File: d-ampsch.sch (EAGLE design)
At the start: 20 parts

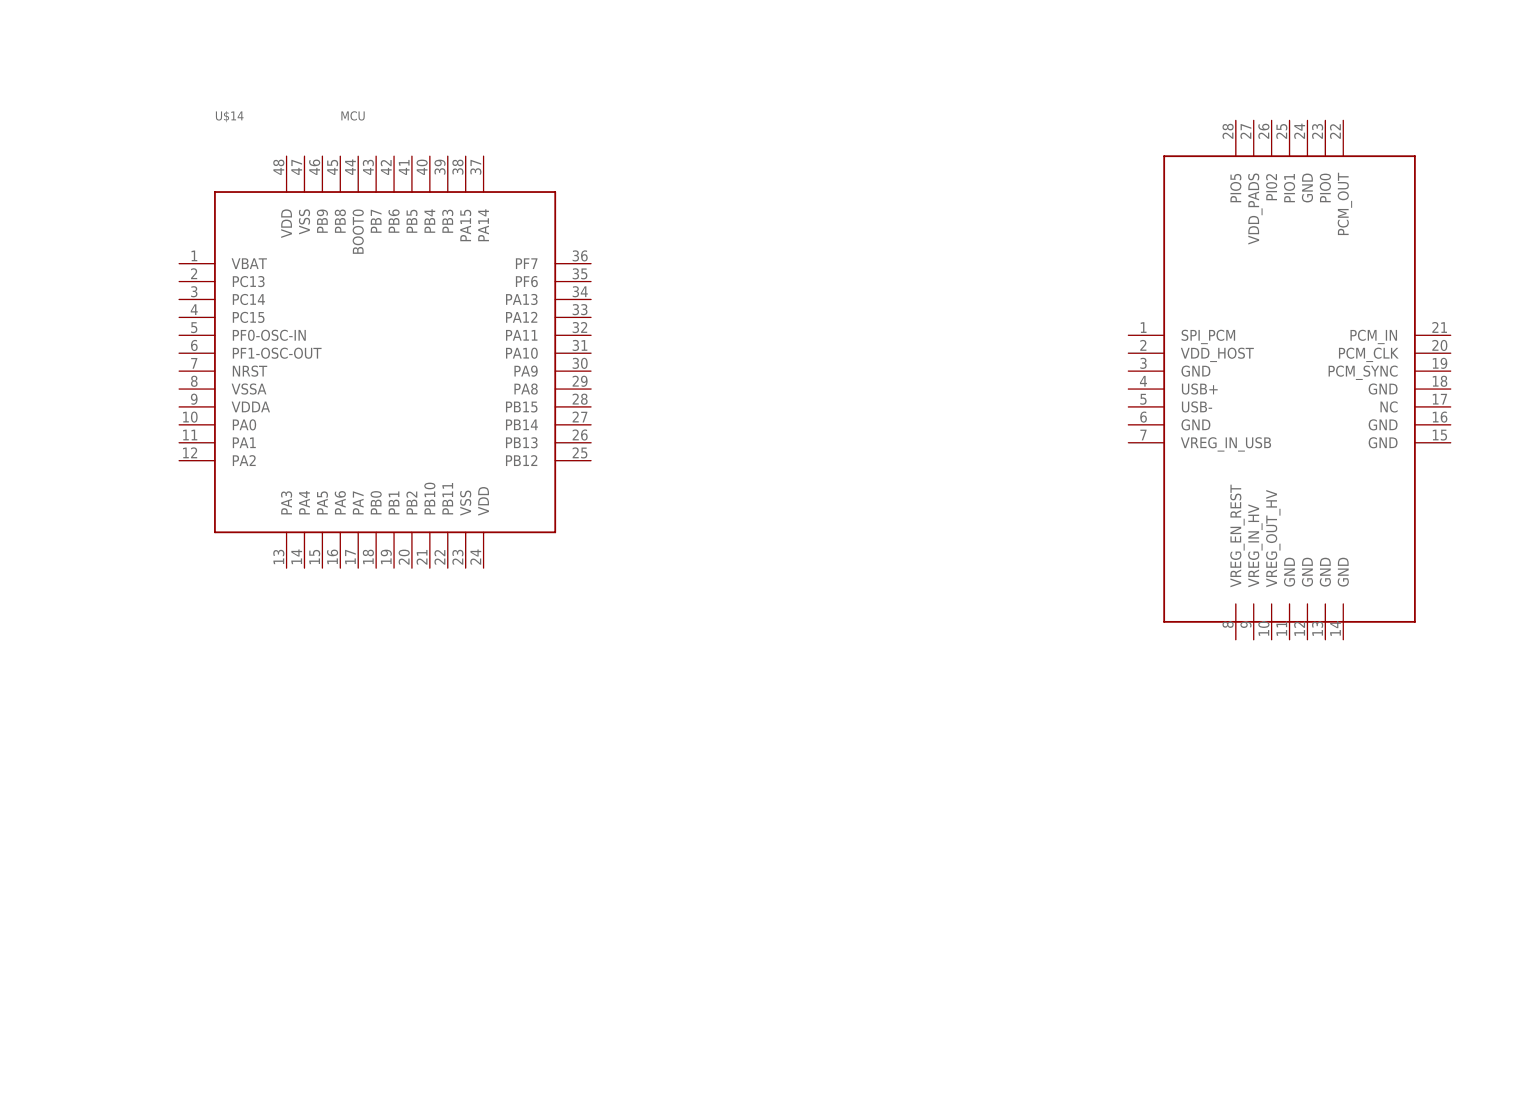
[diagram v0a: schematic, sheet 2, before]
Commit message: updates
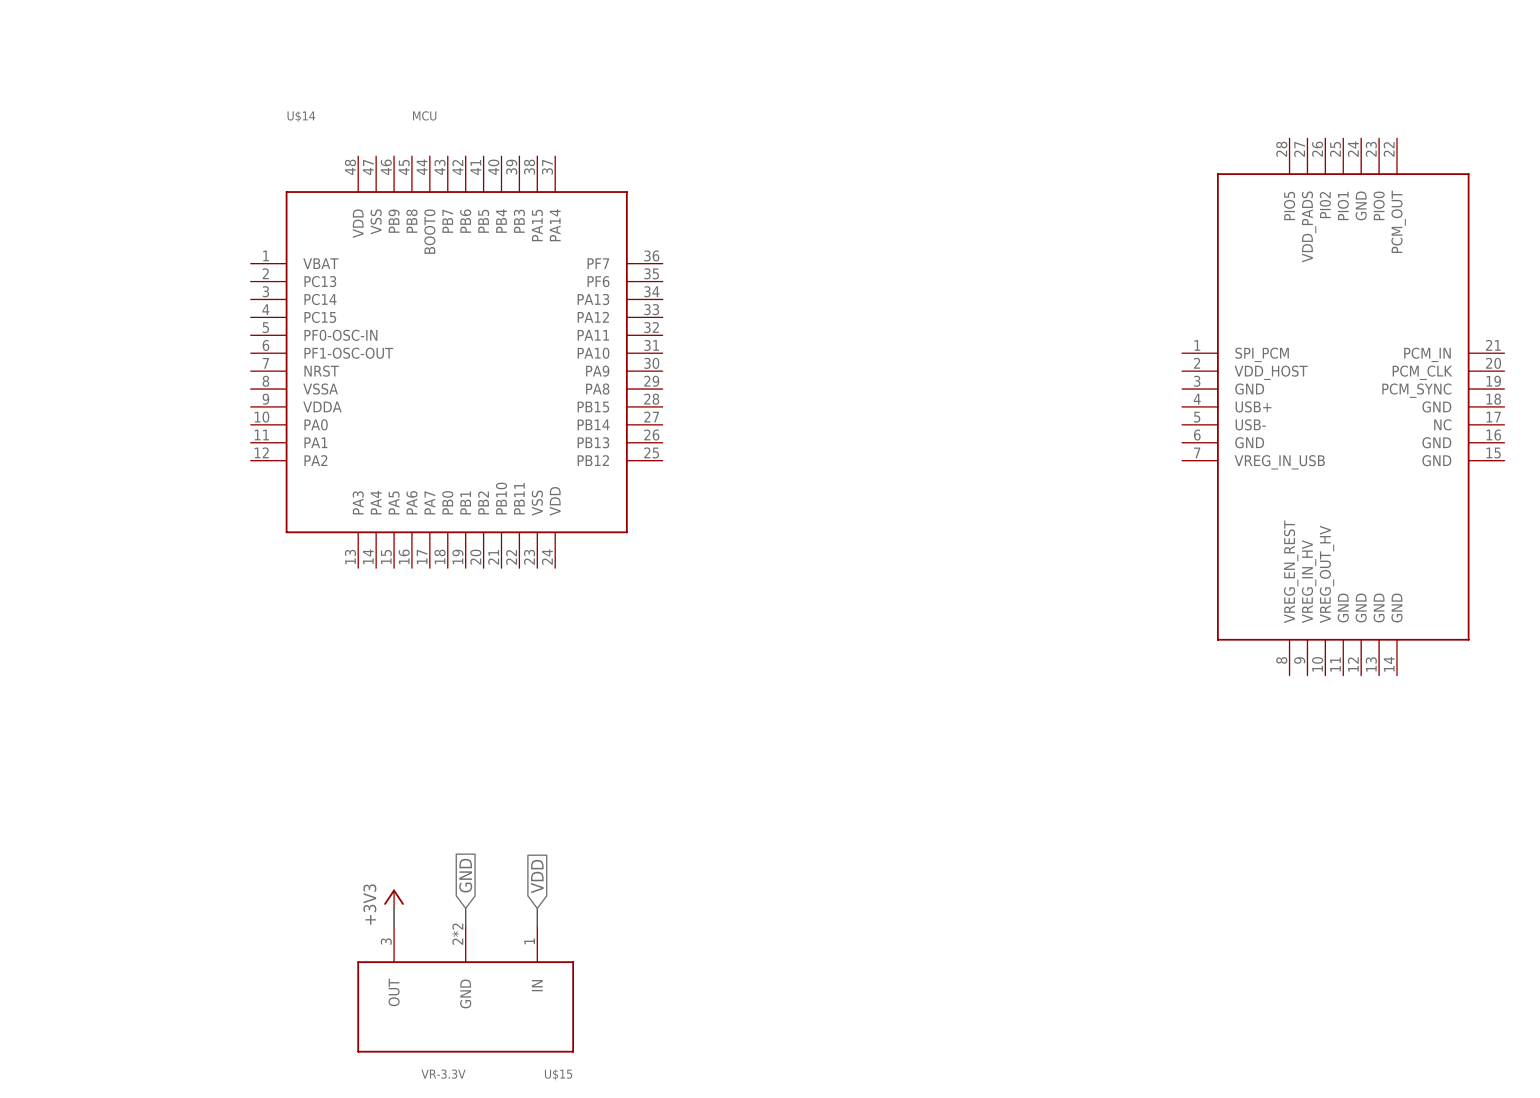
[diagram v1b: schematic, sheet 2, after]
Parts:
- added U$15: VR-3.3V, amplib:VR-3.3V
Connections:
- new net +3V3: U$15.OUT@3
- net GND: now also U$15.GND@24
- net VDD: now also U$15.IN@1
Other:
- moved on the sheet: U$14
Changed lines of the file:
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@@
 <part name="VDD6" library="supply1" library_urn="urn:adsk.eagle:library:371" deviceset="VDD" device=""/>
 <part name="VDD7" library="supply1" library_urn="urn:adsk.eagle:library:371" deviceset="VDD" device=""/>
+<part name="U$14" library="amplib" deviceset="MCU" device="" package3d_urn="urn:adsk.eagle:package:16672024/1"/>
 <part name="U$13" library="amplib" deviceset="BLUETOOTH" device="" package3d_urn="urn:adsk.eagle:package:16526912/1"/>
-<part name="U$14" library="amplib" deviceset="MCU" device="" package3d_urn="urn:adsk.eagle:package:16672024/1"/>
+<part name="U$15" library="amplib" deviceset="VR-3.3V" device="" package3d_urn="urn:adsk.eagle:package:16707660/1"/>
+<part name="+3V1" library="supply1" library_urn="urn:adsk.eagle:library:371" deviceset="+3V3" device=""/>
+<part name="FRAME1" library="frames" library_urn="urn:adsk.eagle:library:229" deviceset="FRAME_B_L" device=""/>
+<part name="FRAME2" library="frames" library_urn="urn:adsk.eagle:library:229" deviceset="FRAME_B_L" device=""/>
 </parts>
 <sheets>
 <sheet>
+<description>D-amp sch</description>
 <plain>
 </plain>
@@
 <instance part="VDD7" gate="G$1" x="40.64" y="10.16" smashed="yes" rot="R270">
 <attribute name="VALUE" x="38.1" y="12.7" size="1.778" layer="96"/>
+</instance>
+<instance part="FRAME1" gate="G$1" x="-106.68" y="-101.6" smashed="yes"/>
+<instance part="FRAME1" gate="G$2" x="218.44" y="-101.6" smashed="yes">
+<attribute name="LAST_DATE_TIME" x="231.14" y="-100.33" size="2.54" layer="94"/>
+<attribute name="SHEET" x="304.8" y="-100.33" size="2.54" layer="94"/>
+<attribute name="DRAWING_NAME" x="236.22" y="-82.55" size="2.54" layer="94"/>
 </instance>
 </instances>
@@
 </sheet>
 <sheet>
+<description>MCU BT SCH</description>
 <plain>
 </plain>
 <instances>
-<instance part="U$13" gate="G$1" x="111.76" y="50.8" smashed="yes"/>
-<instance part="U$14" gate="G$1" x="-30.48" y="53.34" smashed="yes">
-<attribute name="NAME" x="-38.1" y="88.9" size="1.27" layer="95"/>
-<attribute name="VALUE" x="-20.32" y="88.9" size="1.27" layer="96"/>
+<instance part="U$14" gate="G$1" x="-20.32" y="53.34" smashed="yes">
+<attribute name="NAME" x="-27.94" y="88.9" size="1.27" layer="95"/>
+<attribute name="VALUE" x="-10.16" y="88.9" size="1.27" layer="96"/>
+</instance>
+<instance part="U$13" gate="G$1" x="119.38" y="48.26" smashed="yes"/>
+<instance part="U$15" gate="G$1" x="-2.54" y="-35.56" smashed="yes" rot="R180">
+<attribute name="NAME" x="12.7" y="-45.72" size="1.27" layer="95" rot="R180"/>
+<attribute name="VALUE" x="-2.54" y="-45.72" size="1.27" layer="96" rot="R180"/>
+</instance>
+<instance part="+3V1" gate="G$1" x="-12.7" y="-20.32" smashed="yes">
+<attribute name="VALUE" x="-15.24" y="-25.4" size="1.778" layer="96" rot="R90"/>
+</instance>
+<instance part="FRAME2" gate="G$1" x="-132.08" y="-106.68" smashed="yes"/>
+<instance part="FRAME2" gate="G$2" x="193.04" y="-106.68" smashed="yes">
+<attribute name="LAST_DATE_TIME" x="205.74" y="-105.41" size="2.54" layer="94"/>
+<attribute name="SHEET" x="279.4" y="-105.41" size="2.54" layer="94"/>
+<attribute name="DRAWING_NAME" x="210.82" y="-87.63" size="2.54" layer="94"/>
 </instance>
 </instances>
@@
 </busses>
 <nets>
+<net name="GND" class="0">
+<segment>
+<pinref part="U$15" gate="G$1" pin="GND@24"/>
+<wire x1="-2.54" y1="-25.4" x2="-2.54" y2="-22.86" width="0.1524" layer="91"/>
+<label x="-2.54" y="-22.86" size="1.778" layer="95" rot="R90" xref="yes"/>
+</segment>
+</net>
+<net name="+3V3" class="0">
+<segment>
+<pinref part="U$15" gate="G$1" pin="OUT@3"/>
+<wire x1="-12.7" y1="-25.4" x2="-12.7" y2="-22.86" width="0.1524" layer="91"/>
+<pinref part="+3V1" gate="G$1" pin="+3V3"/>
+</segment>
+</net>
+<net name="VDD" class="0">
+<segment>
+<pinref part="U$15" gate="G$1" pin="IN@1"/>
+<wire x1="7.62" y1="-25.4" x2="7.62" y2="-22.86" width="0.1524" layer="91"/>
+<label x="7.62" y="-22.86" size="1.778" layer="95" rot="R90" xref="yes"/>
+</segment>
+</net>
 </nets>
 </sheet>

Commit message: update
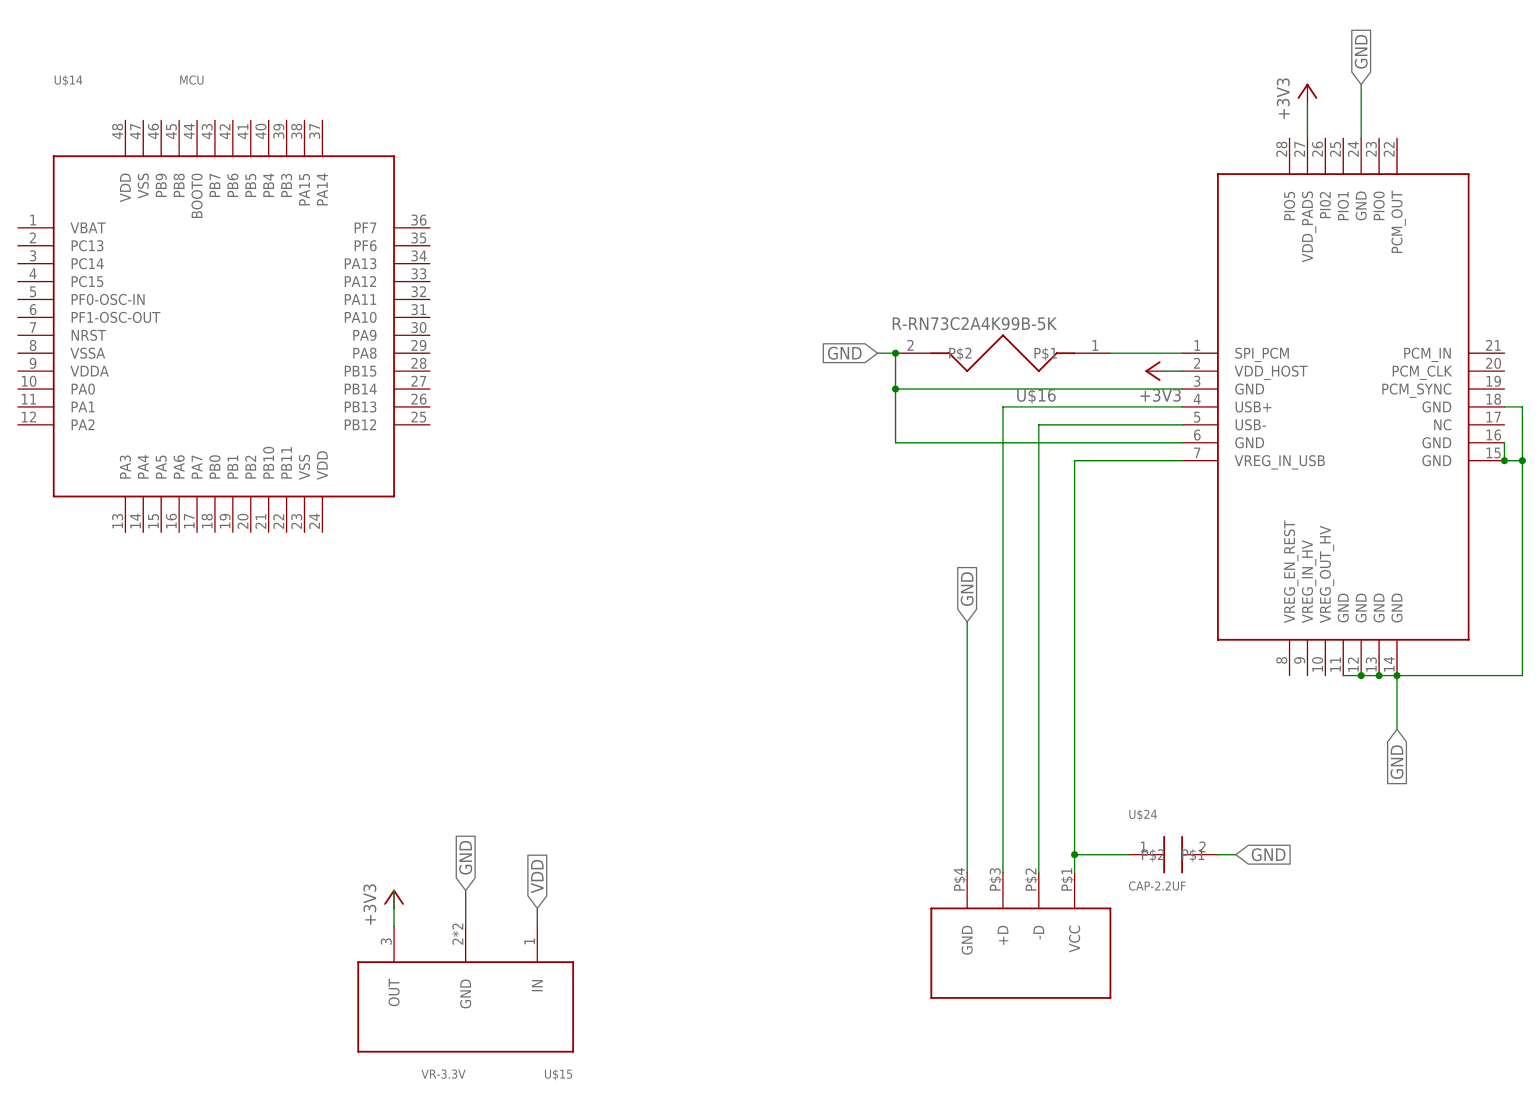
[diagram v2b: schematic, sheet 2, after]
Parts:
- added U$16: R-RN73C2A4K99B-5K, amplib:R-RN73C2A4K99B-5K
- added U$23: USB, amplib:USB
- added U$24: CAP-2.2UF, amplib:CAP-2.2UF
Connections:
- new net N$10: U$13.USB-, U$23.-D@2
- new net N$13: U$13.VREG_IN_USB, U$23.VCC@1, U$24.P$1
- new net N$2: U$13.SPI_PCM, U$16.P$1
- new net N$4: U$13.USB+, U$23.+D@3
- net +3V3: now also U$13.VDD_HOST@2, U$13.VDD_PADS
- net GND: now also U$13.GND@11, U$13.GND@12, U$13.GND@13, U$13.GND@14, U$13.GND@15, U$13.GND@16, U$13.GND@18, U$13.GND@24, U$13.GND@3, U$13.GND@6, U$16.P$2, U$23.GND@4, U$24.P$2
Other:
- moved on the sheet: U$14
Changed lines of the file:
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@@
 <part name="FRAME1" library="frames" library_urn="urn:adsk.eagle:library:229" deviceset="FRAME_B_L" device=""/>
 <part name="FRAME2" library="frames" library_urn="urn:adsk.eagle:library:229" deviceset="FRAME_B_L" device=""/>
+<part name="U$16" library="amplib" deviceset="R-RN73C2A4K99B-5K" device="" package3d_urn="urn:adsk.eagle:package:16497579/1"/>
+<part name="+3V2" library="supply1" library_urn="urn:adsk.eagle:library:371" deviceset="+3V3" device=""/>
+<part name="+3V3" library="supply1" library_urn="urn:adsk.eagle:library:371" deviceset="+3V3" device=""/>
+<part name="U$23" library="amplib" deviceset="USB" device=""/>
+<part name="U$24" library="amplib" deviceset="CAP-2.2UF" device="" package3d_urn="urn:adsk.eagle:package:16732970/1"/>
 </parts>
 <sheets>
@@
 </plain>
 <instances>
-<instance part="U$14" gate="G$1" x="-20.32" y="53.34" smashed="yes">
-<attribute name="NAME" x="-27.94" y="88.9" size="1.27" layer="95"/>
-<attribute name="VALUE" x="-10.16" y="88.9" size="1.27" layer="96"/>
+<instance part="U$14" gate="G$1" x="-53.34" y="58.42" smashed="yes">
+<attribute name="NAME" x="-60.96" y="93.98" size="1.27" layer="95"/>
+<attribute name="VALUE" x="-43.18" y="93.98" size="1.27" layer="96"/>
 </instance>
 <instance part="U$13" gate="G$1" x="119.38" y="48.26" smashed="yes"/>
@@
 <attribute name="DRAWING_NAME" x="210.82" y="-87.63" size="2.54" layer="94"/>
 </instance>
+<instance part="U$16" gate="G$1" x="73.66" y="55.88" smashed="yes" rot="R180">
+<attribute name="NAME" x="81.28" y="50.8" size="1.778" layer="95" rot="R180"/>
+<attribute name="VALUE" x="81.28" y="60.96" size="1.778" layer="96" rot="R180"/>
+</instance>
+<instance part="+3V2" gate="G$1" x="93.98" y="53.34" smashed="yes" rot="R90">
+<attribute name="VALUE" x="99.06" y="50.8" size="1.778" layer="96" rot="R180"/>
+</instance>
+<instance part="+3V3" gate="G$1" x="116.84" y="93.98" smashed="yes">
+<attribute name="VALUE" x="114.3" y="88.9" size="1.778" layer="96" rot="R90"/>
+</instance>
+<instance part="U$23" gate="G$1" x="76.2" y="-22.86" smashed="yes" rot="R180"/>
+<instance part="U$24" gate="G$1" x="99.06" y="-15.24" smashed="yes">
+<attribute name="NAME" x="91.44" y="-10.16" size="1.27" layer="95"/>
+<attribute name="VALUE" x="91.44" y="-20.32" size="1.27" layer="96"/>
+</instance>
 </instances>
 <busses>
@@
 <segment>
 <pinref part="U$15" gate="G$1" pin="GND@24"/>
-<wire x1="-2.54" y1="-25.4" x2="-2.54" y2="-22.86" width="0.1524" layer="91"/>
-<label x="-2.54" y="-22.86" size="1.778" layer="95" rot="R90" xref="yes"/>
+<wire x1="-2.54" y1="-25.4" x2="-2.54" y2="-20.32" width="0.1524" layer="91"/>
+<label x="-2.54" y="-20.32" size="1.778" layer="95" rot="R90" xref="yes"/>
+</segment>
+<segment>
+<pinref part="U$16" gate="G$1" pin="P$2"/>
+<wire x1="58.42" y1="55.88" x2="55.88" y2="55.88" width="0.1524" layer="91"/>
+<pinref part="U$13" gate="G$1" pin="GND@3"/>
+<wire x1="99.06" y1="50.8" x2="58.42" y2="50.8" width="0.1524" layer="91"/>
+<wire x1="58.42" y1="50.8" x2="58.42" y2="55.88" width="0.1524" layer="91"/>
+<junction x="58.42" y="55.88"/>
+<pinref part="U$13" gate="G$1" pin="GND@6"/>
+<wire x1="99.06" y1="43.18" x2="58.42" y2="43.18" width="0.1524" layer="91"/>
+<wire x1="58.42" y1="43.18" x2="58.42" y2="50.8" width="0.1524" layer="91"/>
+<junction x="58.42" y="50.8"/>
+<label x="55.88" y="55.88" size="1.778" layer="95" rot="R180" xref="yes"/>
+</segment>
+<segment>
+<pinref part="U$13" gate="G$1" pin="GND@18"/>
+<wire x1="144.78" y1="48.26" x2="147.32" y2="48.26" width="0.1524" layer="91"/>
+<wire x1="147.32" y1="48.26" x2="147.32" y2="40.64" width="0.1524" layer="91"/>
+<pinref part="U$13" gate="G$1" pin="GND@15"/>
+<wire x1="147.32" y1="40.64" x2="144.78" y2="40.64" width="0.1524" layer="91"/>
+<pinref part="U$13" gate="G$1" pin="GND@16"/>
+<wire x1="144.78" y1="43.18" x2="144.78" y2="40.64" width="0.1524" layer="91"/>
+<junction x="144.78" y="40.64"/>
+<pinref part="U$13" gate="G$1" pin="GND@11"/>
+<pinref part="U$13" gate="G$1" pin="GND@14"/>
+<wire x1="121.92" y1="10.16" x2="124.46" y2="10.16" width="0.1524" layer="91"/>
+<pinref part="U$13" gate="G$1" pin="GND@12"/>
+<wire x1="124.46" y1="10.16" x2="127" y2="10.16" width="0.1524" layer="91"/>
+<junction x="124.46" y="10.16"/>
+<pinref part="U$13" gate="G$1" pin="GND@13"/>
+<wire x1="127" y1="10.16" x2="129.54" y2="10.16" width="0.1524" layer="91"/>
+<junction x="127" y="10.16"/>
+<wire x1="129.54" y1="10.16" x2="129.54" y2="2.54" width="0.1524" layer="91"/>
+<junction x="129.54" y="10.16"/>
+<wire x1="147.32" y1="40.64" x2="147.32" y2="10.16" width="0.1524" layer="91"/>
+<wire x1="147.32" y1="10.16" x2="129.54" y2="10.16" width="0.1524" layer="91"/>
+<junction x="147.32" y="40.64"/>
+<label x="129.54" y="2.54" size="1.778" layer="95" rot="R270" xref="yes"/>
+</segment>
+<segment>
+<pinref part="U$13" gate="G$1" pin="GND@24"/>
+<wire x1="124.46" y1="86.36" x2="124.46" y2="93.98" width="0.1524" layer="91"/>
+<label x="124.46" y="93.98" size="1.778" layer="95" rot="R90" xref="yes"/>
+</segment>
+<segment>
+<pinref part="U$23" gate="G$1" pin="GND@4"/>
+<wire x1="68.58" y1="-17.78" x2="68.58" y2="17.78" width="0.1524" layer="91"/>
+<label x="68.58" y="17.78" size="1.778" layer="95" rot="R90" xref="yes"/>
+</segment>
+<segment>
+<pinref part="U$24" gate="G$1" pin="P$2"/>
+<wire x1="104.14" y1="-15.24" x2="106.68" y2="-15.24" width="0.1524" layer="91"/>
+<label x="106.68" y="-15.24" size="1.778" layer="95" xref="yes"/>
 </segment>
 </net>
@@
 <wire x1="-12.7" y1="-25.4" x2="-12.7" y2="-22.86" width="0.1524" layer="91"/>
 <pinref part="+3V1" gate="G$1" pin="+3V3"/>
+<wire x1="-12.7" y1="-22.86" x2="-12.7" y2="-20.32" width="0.1524" layer="91"/>
+</segment>
+<segment>
+<pinref part="+3V2" gate="G$1" pin="+3V3"/>
+<pinref part="U$13" gate="G$1" pin="VDD_HOST@2"/>
+<wire x1="96.52" y1="53.34" x2="99.06" y2="53.34" width="0.1524" layer="91"/>
+</segment>
+<segment>
+<pinref part="U$13" gate="G$1" pin="VDD_PADS"/>
+<pinref part="+3V3" gate="G$1" pin="+3V3"/>
+<wire x1="116.84" y1="86.36" x2="116.84" y2="91.44" width="0.1524" layer="91"/>
 </segment>
 </net>
@@
 </segment>
 </net>
+<net name="N$2" class="0">
+<segment>
+<pinref part="U$16" gate="G$1" pin="P$1"/>
+<pinref part="U$13" gate="G$1" pin="SPI_PCM"/>
+<wire x1="88.9" y1="55.88" x2="99.06" y2="55.88" width="0.1524" layer="91"/>
+</segment>
+</net>
+<net name="N$4" class="0">
+<segment>
+<pinref part="U$13" gate="G$1" pin="USB+"/>
+<wire x1="99.06" y1="48.26" x2="73.66" y2="48.26" width="0.1524" layer="91"/>
+<pinref part="U$23" gate="G$1" pin="+D@3"/>
+<wire x1="73.66" y1="48.26" x2="73.66" y2="-17.78" width="0.1524" layer="91"/>
+</segment>
+</net>
+<net name="N$10" class="0">
+<segment>
+<pinref part="U$13" gate="G$1" pin="USB-"/>
+<wire x1="99.06" y1="45.72" x2="78.74" y2="45.72" width="0.1524" layer="91"/>
+<pinref part="U$23" gate="G$1" pin="-D@2"/>
+<wire x1="78.74" y1="45.72" x2="78.74" y2="-17.78" width="0.1524" layer="91"/>
+</segment>
+</net>
+<net name="N$13" class="0">
+<segment>
+<pinref part="U$13" gate="G$1" pin="VREG_IN_USB"/>
+<wire x1="99.06" y1="40.64" x2="83.82" y2="40.64" width="0.1524" layer="91"/>
+<pinref part="U$23" gate="G$1" pin="VCC@1"/>
+<wire x1="83.82" y1="40.64" x2="83.82" y2="-15.24" width="0.1524" layer="91"/>
+<pinref part="U$24" gate="G$1" pin="P$1"/>
+<wire x1="83.82" y1="-15.24" x2="83.82" y2="-17.78" width="0.1524" layer="91"/>
+<wire x1="91.44" y1="-15.24" x2="83.82" y2="-15.24" width="0.1524" layer="91"/>
+<junction x="83.82" y="-15.24"/>
+</segment>
+</net>
